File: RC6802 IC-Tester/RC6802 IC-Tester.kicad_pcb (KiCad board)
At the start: 2 copper layers, 99.1 x 86.4 mm, 80 parts, among them J1 TAPE, J2 RC6802_UI_Port, J3 EXT_KEYPAD, M1 Mounting, M2 Mounting, M3 Mounting, M4 Mounting, Q1 2N3906, Q2 2N3906, Q3 2N3904, Q4 2N3904, Q5 2N3904, SW1 RESET, SW10 D, SW11 2, SW12 6, SW13 A, SW14 E, SW15 3, SW16 7, SW17 B, SW18 F, SW19 TAPE, SW2 ~IRQ, SW20 STEP, SW21 SST, SW3 Ø, SW4 4, SW5 8, SW6 C, SW7 1, SW8 5, SW9 9, U1 74LS374, U2 74LS00, U3 74LS73

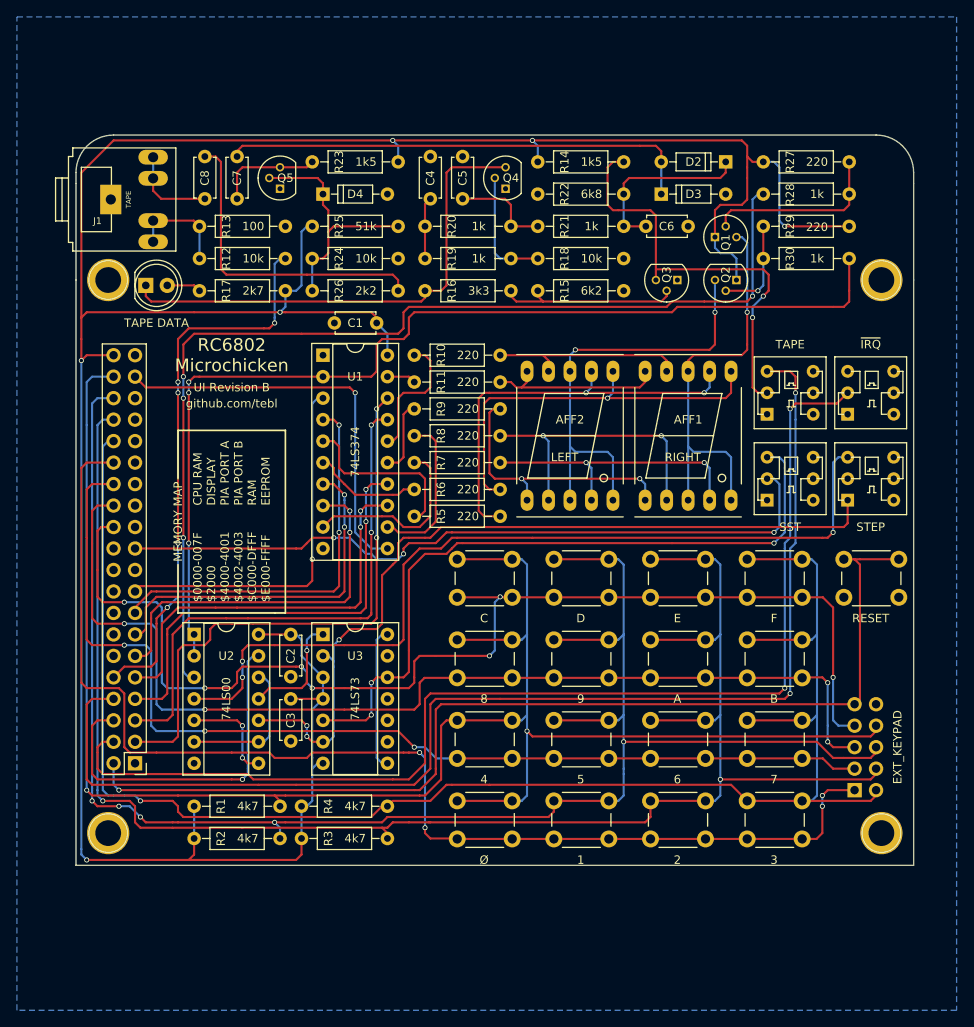
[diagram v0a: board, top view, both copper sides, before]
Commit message: IC-Tester layout
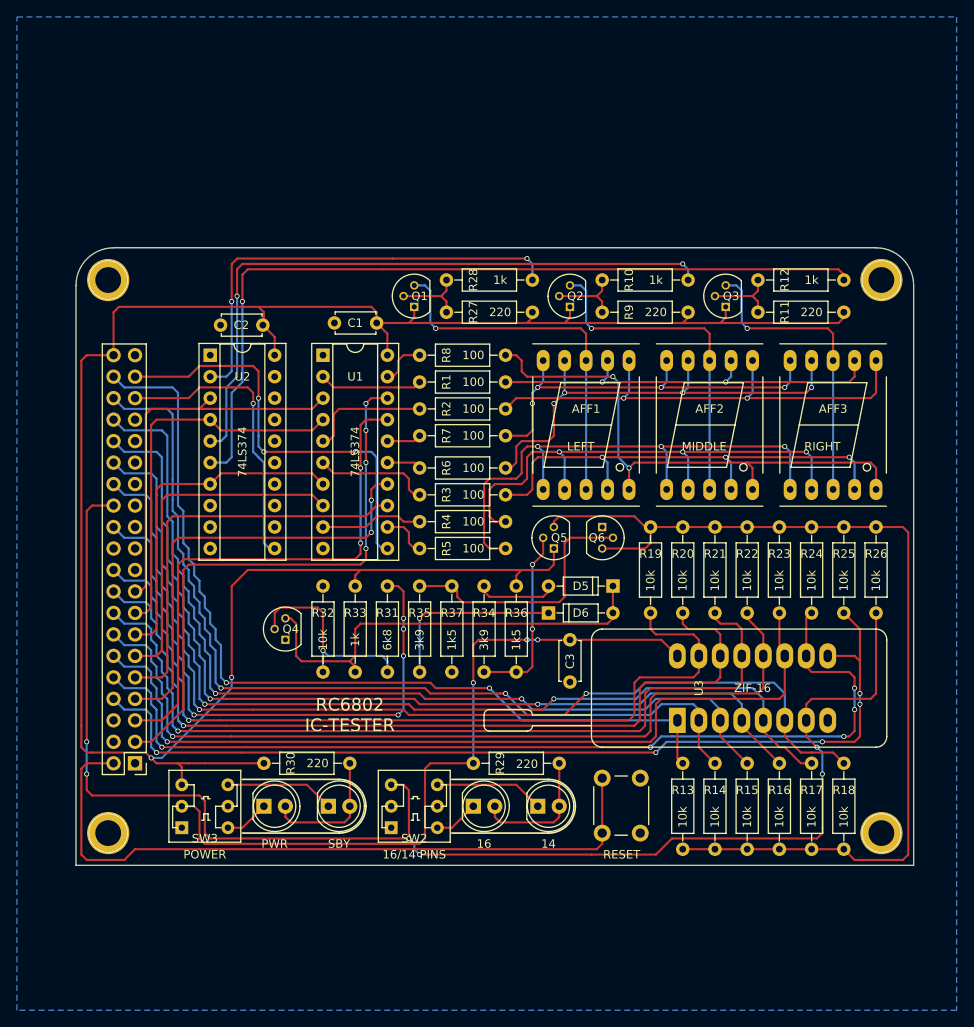
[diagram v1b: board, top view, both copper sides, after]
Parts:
- removed C4, C6: 50nF, Capacitors_THT:C_Disc_D4.7mm_W2.5mm_P5.00mm
- removed C5: 68nF, Capacitors_THT:C_Disc_D4.7mm_W2.5mm_P5.00mm
- removed C7: 500nF, Capacitors_THT:C_Disc_D4.7mm_W2.5mm_P5.00mm
- removed C8: 100nF, Capacitors_THT:C_Disc_D4.7mm_W2.5mm_P5.00mm
- removed J1: TAPE, TRS:Tayda_3.5mm_stereo_TRS_jack_A-853
- removed J3: EXT_KEYPAD, Pin_Headers:Pin_Header_Angled_2x05_Pitch2.54mm
- removed SW10: D, Buttons_Switches_THT:SW_PUSH_6mm
- removed SW11: 2, Buttons_Switches_THT:SW_PUSH_6mm
- removed SW12: 6, Buttons_Switches_THT:SW_PUSH_6mm
- removed SW13: A, Buttons_Switches_THT:SW_PUSH_6mm
- removed SW14: E, Buttons_Switches_THT:SW_PUSH_6mm
- removed SW15: 3, Buttons_Switches_THT:SW_PUSH_6mm
- removed SW16: 7, Buttons_Switches_THT:SW_PUSH_6mm
- removed SW17: B, Buttons_Switches_THT:SW_PUSH_6mm
- removed SW18: F, Buttons_Switches_THT:SW_PUSH_6mm
- removed SW19: TAPE, DPDT_Switch:dpdt_switch
- removed SW20: STEP, DPDT_Switch:dpdt_switch
- removed SW21: SST, DPDT_Switch:dpdt_switch
- removed SW4: 4, Buttons_Switches_THT:SW_PUSH_6mm
- removed SW5: 8, Buttons_Switches_THT:SW_PUSH_6mm
- removed SW6: C, Buttons_Switches_THT:SW_PUSH_6mm
- removed SW7: 1, Buttons_Switches_THT:SW_PUSH_6mm
- removed SW8: 5, Buttons_Switches_THT:SW_PUSH_6mm
- removed SW9: 9, Buttons_Switches_THT:SW_PUSH_6mm
- added AFF3: RIGHT, Displays_7-Segment:7SegmentLED_LTS6760_LTS6780, F.Cu at (189.9, 92.1)
- added D5: 1N4148, Diodes_THT:D_DO-35_SOD27_P7.62mm_Horizontal, F.Cu at (163.8, 111.1)
- added D6: 1N4148, Diodes_THT:D_DO-35_SOD27_P7.62mm_Horizontal, F.Cu at (156.2, 114.3)
- added Q6: 2N3904, TO_SOT_Packages_THT:TO-92_Molded_Narrow, F.Cu at (162.6, 104.1)
- added R31: 6k8, Resistors_THT:R_Axial_DIN0207_L6.3mm_D2.5mm_P10.16mm_Horizontal, F.Cu at (137.2, 111.1)
- added R32: 10k, Resistors_THT:R_Axial_DIN0207_L6.3mm_D2.5mm_P10.16mm_Horizontal, F.Cu at (129.5, 111.1)
- added R33: 1k, Resistors_THT:R_Axial_DIN0207_L6.3mm_D2.5mm_P10.16mm_Horizontal, F.Cu at (133.3, 111.1)
- added R34: 3k9, Resistors_THT:R_Axial_DIN0207_L6.3mm_D2.5mm_P10.16mm_Horizontal, F.Cu at (148.6, 121.3)
- added R35: 3k9, Resistors_THT:R_Axial_DIN0207_L6.3mm_D2.5mm_P10.16mm_Horizontal, F.Cu at (141.0, 121.3)
- added R36: 1k5, Resistors_THT:R_Axial_DIN0207_L6.3mm_D2.5mm_P10.16mm_Horizontal, F.Cu at (152.4, 111.1)
- added R37: 1k5, Resistors_THT:R_Axial_DIN0207_L6.3mm_D2.5mm_P10.16mm_Horizontal, F.Cu at (144.8, 121.3)
- AFF1: value RIGHT -> LEFT
- AFF2: value LEFT -> MIDDLE
- D1: value DATA_IN -> 14
- D2: value 1n914 -> 16; footprint Diodes_THT:D_DO-35_SOD27_P7.62mm_Horizontal -> LEDs:LED_D5.0mm
- D3: value 1n914 -> SBY; footprint Diodes_THT:D_DO-35_SOD27_P7.62mm_Horizontal -> LEDs:LED_D5.0mm
- D4: value 1n914 -> PWR; footprint Diodes_THT:D_DO-35_SOD27_P7.62mm_Horizontal -> LEDs:LED_D5.0mm
- Q3, Q5: value 2N3904 -> 2N3906
- R1, R2, R3, R4: value 4k7 -> 100
- R10: value 220 -> 1k
- R12: value 10k -> 1k
- R13: value 100 -> 10k
- R14, R23: value 1k5 -> 10k
- R15: value 6k2 -> 10k
- R16: value 3k3 -> 10k
- R17: value 2k7 -> 10k
- R19, R20, R21: value 1k -> 10k
- R22: value 6k8 -> 10k
- R25: value 51k -> 10k
- R26: value 2k2 -> 10k
- R30: value 1k -> 220
- R5, R6, R7, R8: value 220 -> 100
- SW2: value ~IRQ -> PINS; footprint DPDT_Switch:dpdt_switch -> DPDT_Switch:dpdt_switch_black
- SW3: value Ø -> ZIF_PWR; footprint Buttons_Switches_THT:SW_PUSH_6mm -> DPDT_Switch:dpdt_switch_black
- U2: value 74LS00 -> 74LS374; footprint Housings_DIP:DIP-14_W7.62mm_Socket -> Housings_DIP:DIP-20_W7.62mm_Socket
- U3: value 74LS73 -> ZIF-16; footprint Housings_DIP:DIP-14_W7.62mm_Socket -> ZIF:ZIF-16
- moved R17 91.4 mm to (187.3, 132.1), turned to 270 degrees
- moved R13 85.4 mm to (172.1, 132.1), turned to 270 degrees
- moved R30 84.0 mm to (122.6, 132.1)
- moved D3 82.4 mm to (130.2, 137.2)
- moved D2 81.8 mm to (147.3, 137.2), turned to 0 degrees
- moved D1 77.1 mm to (154.9, 137.2)
- moved R26 76.8 mm to (194.9, 114.3), turned to 90 degrees
- moved R12 76.2 mm to (191.1, 74.9), turned to 180 degrees
- moved SW2 72.8 mm to (140.3, 137.2)
- moved D4 72.7 mm to (122.6, 137.2)
- moved R25 72.2 mm to (191.1, 104.1), turned to 270 degrees
- moved R29 72.2 mm to (147.3, 132.1)
- moved R14 71.9 mm to (175.9, 132.1), turned to 270 degrees
- moved R23 70.1 mm to (183.5, 104.1), turned to 270 degrees
- moved R16 69.8 mm to (183.5, 132.1), turned to 270 degrees
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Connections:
- AFF1 pad 5: Net-(AFF1-Pad3) -> Net-(AFF1-Pad5)
- AFF2 pad 5: Net-(AFF2-Pad3) -> Net-(AFF1-Pad5)
- C3 pad 1: VCC -> Net-(C3-Pad1)
- D2 pad 1: Net-(C6-Pad2) -> Net-(D2-Pad1)
- D2 pad 2: Net-(C7-Pad1) -> Net-(D1-Pad2)
- D3 pad 1: Net-(C7-Pad1) -> Net-(D3-Pad1)
- D3 pad 2: GND -> Net-(D3-Pad2)
- D4 pad 2: GND -> Net-(D3-Pad2)
- J2 pad 12: (no net) -> /PB5
- J2 pad 14: (no net) -> /PB4
- J2 pad 16: (no net) -> /PB3
- J2 pad 18: (no net) -> /PB2
- J2 pad 20: (no net) -> /PB1
- J2 pad 21: /~HALT -> (no net)
- J2 pad 35: (no net) -> /IO1
- J2 pad 4: ~SST -> (no net)
- J2 pad 6: /E -> (no net)
- Q3 pad 1: GND -> VCC
- Q3 pad 3: Net-(Q3-Pad3) -> Net-(AFF3-Pad3)
- Q4 pad 3: Net-(D1-Pad1) -> Net-(D5-Pad1)
- Q5 pad 1: GND -> VCC
- Q5 pad 2: Net-(D4-Pad1) -> Net-(Q5-Pad2)
- Q5 pad 3: Net-(C7-Pad2) -> Net-(Q5-Pad3)
- R1 pad 1: VCC -> Net-(AFF1-Pad7)
- R1 pad 2: /PA0 -> Net-(R1-Pad2)
- R10 pad 1: Net-(AFF1-Pad9) -> Net-(R10-Pad1)
- R10 pad 2: Net-(R10-Pad2) -> Net-(Q2-Pad2)
- R11 pad 1: Net-(AFF1-Pad10) -> VCC
- R11 pad 2: Net-(R11-Pad2) -> Net-(Q3-Pad2)
- R12 pad 1: /TAPE_MIC -> Net-(R12-Pad1)
- R12 pad 2: /PB6 -> Net-(Q3-Pad2)
- R13 pad 1: /TAPE_MIC -> /PA0
- R13 pad 2: GND -> Net-(Q5-Pad3)
- R14 pad 1: Net-(Q3-Pad3) -> /PA1
- R14 pad 2: VCC -> Net-(Q5-Pad3)
- R15 pad 1: Net-(Q3-Pad2) -> /PA2
- R15 pad 2: GND -> Net-(Q5-Pad3)
- R16 pad 1: Net-(D1-Pad1) -> /PA3
- R16 pad 2: Net-(Q3-Pad2) -> Net-(Q5-Pad3)
- R17 pad 1: Net-(D1-Pad2) -> /PA4
- R17 pad 2: VCC -> Net-(Q5-Pad3)
- R18 pad 1: GND -> /PA5
- R18 pad 2: Net-(Q4-Pad2) -> Net-(Q5-Pad3)
- R19 pad 1: Net-(C4-Pad2) -> Net-(Q5-Pad3)
- R19 pad 2: Net-(Q4-Pad2) -> /PB1
- R2 pad 1: VCC -> Net-(AFF1-Pad6)
- R2 pad 2: /PA1 -> Net-(R2-Pad2)
- R20 pad 1: Net-(C5-Pad2) -> Net-(Q5-Pad3)
- R20 pad 2: Net-(C4-Pad2) -> /PB2
- R21 pad 1: Net-(C6-Pad2) -> Net-(Q5-Pad3)
- R21 pad 2: Net-(C5-Pad2) -> /PB3
- R22 pad 1: Net-(C6-Pad2) -> Net-(Q5-Pad3)
- R22 pad 2: GND -> /PB4
- R23 pad 1: Net-(C7-Pad2) -> Net-(Q5-Pad3)
- R23 pad 2: VCC -> /PB5
- R24 pad 1: Net-(D4-Pad1) -> Net-(Q5-Pad3)
- R24 pad 2: GND -> /PB6
- R25 pad 1: VCC -> Net-(Q5-Pad3)
- R25 pad 2: Net-(D4-Pad1) -> /PB7
- R26 pad 1: Net-(D4-Pad1) -> /PA6
- R26 pad 2: Net-(C8-Pad1) -> Net-(Q5-Pad3)
- R29 pad 1: Net-(Q2-Pad2) -> Net-(C3-Pad1)
- R29 pad 2: VCC -> Net-(D1-Pad2)
- R3 pad 1: VCC -> Net-(AFF1-Pad4)
- R3 pad 2: /PA2 -> Net-(R3-Pad2)
- R30 pad 1: Net-(Q2-Pad2) -> VCC
- R30 pad 2: Net-(R30-Pad2) -> Net-(D3-Pad2)
- R4 pad 1: VCC -> Net-(AFF1-Pad2)
- R4 pad 2: /PA3 -> Net-(R4-Pad2)
- R5 pad 1: Net-(AFF1-Pad7) -> Net-(AFF1-Pad1)
- R6 pad 1: Net-(AFF1-Pad6) -> Net-(AFF1-Pad9)
- R7 pad 1: Net-(AFF1-Pad4) -> Net-(AFF1-Pad10)
- R8 pad 1: Net-(AFF1-Pad2) -> Net-(AFF1-Pad5)
- R9 pad 1: Net-(AFF1-Pad1) -> VCC
- R9 pad 2: Net-(R9-Pad2) -> Net-(Q2-Pad2)
- SW2 pad 2: ~SST -> GND
- SW2 pad 3: GND -> /PA6
- SW2 pad 4: (no net) -> Net-(D2-Pad1)
- SW2 pad 5: (no net) -> GND
- SW2 pad 6: (no net) -> Net-(D1-Pad1)
- SW3 pad 1: /PA0 -> (no net)
- SW3 pad 2: /PA4 -> Net-(C3-Pad1)
- U1 pad 12: Net-(R8-Pad2) -> Net-(R5-Pad2)
- U1 pad 15: Net-(R9-Pad2) -> Net-(R6-Pad2)
- U1 pad 16: Net-(R10-Pad2) -> Net-(R7-Pad2)
- U1 pad 19: Net-(R11-Pad2) -> Net-(R8-Pad2)
- U1 pad 2: Net-(R30-Pad2) -> Net-(R1-Pad2)
- U1 pad 5: Net-(R5-Pad2) -> Net-(R2-Pad2)
- U1 pad 6: Net-(R6-Pad2) -> Net-(R3-Pad2)
- U1 pad 9: Net-(R7-Pad2) -> Net-(R4-Pad2)
- U2 pad 1: Net-(R30-Pad2) -> GND
- U2 pad 10: Net-(SW20-Pad1) -> GND
- U2 pad 11: Net-(U2-Pad11) -> /IO1
- U2 pad 12: Net-(U2-Pad12) -> (no net)
- U2 pad 13: /E -> GND
- U2 pad 14: VCC -> GND
- U2 pad 2: Net-(R30-Pad2) -> Net-(R28-Pad1)
- U2 pad 3: Net-(R28-Pad1) -> /D0
- U2 pad 4: Net-(SW20-Pad3) -> /D1
- U2 pad 5: Net-(U2-Pad5) -> Net-(R10-Pad1)
- U2 pad 6: Net-(U2-Pad12) -> Net-(R12-Pad1)
- U2 pad 7: GND -> /D2
- U2 pad 8: Net-(U2-Pad5) -> GND
- U2 pad 9: Net-(U2-Pad12) -> (no net)
- U3 pad 1: Net-(U2-Pad11) -> /PA0
- U3 pad 10: GND -> /PB6
- U3 pad 11: GND -> /PB5
- U3 pad 12: Net-(SW21-Pad3) -> /PB4
- U3 pad 13: (no net) -> /PB3
- U3 pad 14: Net-(U3-Pad14) -> /PB2
- U3 pad 2: Net-(SW20-Pad1) -> /PA1
- U3 pad 3: VCC -> /PA2
- U3 pad 4: VCC -> /PA3
- U3 pad 5: Net-(SW21-Pad3) -> /PA4
- U3 pad 6: Net-(SW20-Pad1) -> /PA5
- U3 pad 7: VCC -> /PA6
- U3 pad 8: Net-(U3-Pad14) -> GND
- U3 pad 9: (no net) -> /PB7
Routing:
- net ~SST: track 137.0 -> 0.00 mm, vias 2 -> 0
- net Net-(R30-Pad2): track 122.8 -> 0.00 mm, vias 3 -> 0
- net Net-(Q5-Pad3): track 0.00 -> 117.0 mm
- net /PA0: track 209.2 -> 105.6 mm
- net Net-(SW20-Pad3): track 101.8 -> 0.00 mm, vias 3 -> 0
- net /PB5: track 0.00 -> 101.7 mm, vias 0 -> 1
- net /PB2: track 0.00 -> 101.1 mm, vias 0 -> 1
- net /PB4: track 0.00 -> 100.6 mm, vias 0 -> 1
- net /PB3: track 0.00 -> 100.6 mm, vias 0 -> 1
- net /PB1: track 0.00 -> 99.8 mm, vias 0 -> 1
- net Net-(SW20-Pad1): track 97.8 -> 0.00 mm, vias 3 -> 0
- net Net-(R12-Pad1): track 0.00 -> 97.2 mm, vias 0 -> 1
- net /PA1: track 202.3 -> 108.3 mm, vias 5 -> 2
- net /PA2: track 198.7 -> 109.2 mm
- net /~HALT: track 86.5 -> 0.00 mm, vias 3 -> 0
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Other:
- board size 99.1 x 86.4 mm -> 99.1 x 73 mm
- board text added: "$2400"
- board text added: "16/14 PINS"
- board text added: "DISPLAY CONTROL"
- board text added: "POWER"
- board text added: "RC6802 IC-TESTER"
- board text added: "RESET"
- board text added: "SEGMENT OUTPUT"
- board text removed: "$0000-007F $2000 $4000-4001 $4002-4003 $C000-DFFF $E000-FFFF"
- board text removed: "$FFFE $FFFC $FFFA $FFF8"
- board text removed: "$FFFF $FFFD $FFFB $FFF9"
- board text removed: "1 0001"
- board text removed: "2 0010"
- board text removed: "3 0011"
- board text removed: "4 0100"
- board text removed: "5 0101"
- board text removed: "6 0110"
- board text removed: "7 0111"
- board text removed: "8 1000"
- board text removed: "9 1001"
- board text removed: "A 1010"
- board text removed: "B 1011"
- board text removed: "C 1100"
- board text removed: "C.A."
- board text removed: "CPU RAM DISPLAY PIA PORT A PIA PORT B RAM EEPROM"
- board text removed: "D 1101"
- board text removed: "DATA OUTPUT LATCH"
- board text removed: "E 1110"
- board text removed: "F 1111"
- board text removed: "HEX KEYPAD"
- board text removed: "HW SST"
- board text removed: "INTERRUPT VECTORS"
- board text removed: "JK FLIP-FLOP"
- board text removed: "LS"
- board text removed: "MEMORY MAP"
- board text removed: "MS"
- board text removed: "NAND GATES"
- board text removed: "RC6802 Microchicken"
- board text removed: "RESTART NON-MASKABLE INT. SOFTWARE INTERRUPT INTERRUPT REQUEST"
- board text removed: "TAPE DATA"
- board text removed: "TAPE INPUT/OUTPUT"
- board text removed: "UI Revision B"
- board text removed: "github.com/tebl"
- board text removed: "Ø 0000"
